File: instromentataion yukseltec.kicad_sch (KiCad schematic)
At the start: 0 parts

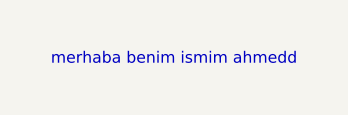
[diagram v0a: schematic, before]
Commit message: aa
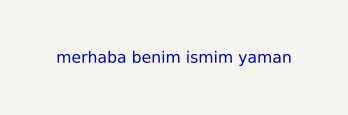
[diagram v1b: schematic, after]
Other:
- note added: "merhaba benim ismim yaman"
- note removed: "merhaba benim ismim ahmedd"
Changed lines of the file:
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@@
 	(generator_version "10.0")
 	(paper "A4")
-	(text "merhaba benim ismim ahmedd"
+	(text "merhaba benim ismim yaman"
 		(exclude_from_sim no)
 		(at 139.7 95.25 0)

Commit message: Revert "aa"
This reverts commit af853fb5f618a00eec8f8c9e7ae50b6d576ae841.
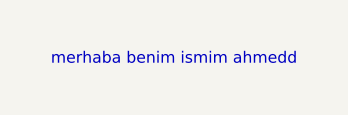
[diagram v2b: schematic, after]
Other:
- note added: "merhaba benim ismim ahmedd"
- note removed: "merhaba benim ismim yaman"
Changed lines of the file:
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@@
 	(generator_version "10.0")
 	(paper "A4")
-	(text "merhaba benim ismim yaman"
+	(text "merhaba benim ismim ahmedd"
 		(exclude_from_sim no)
 		(at 139.7 95.25 0)

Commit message: kardes_napyon_eklendi
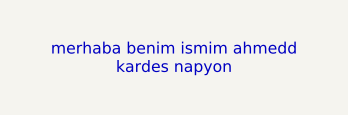
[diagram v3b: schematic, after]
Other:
- note added: "merhaba benim ismim ahmedd kardes napyon"
- note removed: "merhaba benim ismim ahmedd"
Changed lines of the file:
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@@
 	(generator_version "10.0")
 	(paper "A4")
-	(text "merhaba benim ismim ahmedd"
+	(text "merhaba benim ismim ahmedd\nkardes napyon"
 		(exclude_from_sim no)
 		(at 139.7 95.25 0)

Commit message: red_yedik
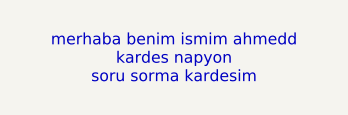
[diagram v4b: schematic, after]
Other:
- note added: "merhaba benim ismim ahmedd kardes napyon soru sorma kardesim"
- note removed: "merhaba benim ismim ahmedd kardes napyon"
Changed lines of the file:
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@@
 	(generator_version "10.0")
 	(paper "A4")
-	(text "merhaba benim ismim ahmedd\nkardes napyon"
+	(text "merhaba benim ismim ahmedd\nkardes napyon\nsoru sorma kardesim"
 		(exclude_from_sim no)
 		(at 139.7 95.25 0)

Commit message: ozur
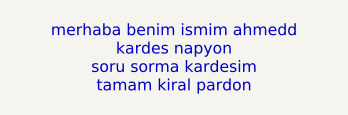
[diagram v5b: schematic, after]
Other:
- note added: "merhaba benim ismim ahmedd kardes napyon soru sorma kardesim tamam kiral pardon"
- note removed: "merhaba benim ismim ahmedd kardes napyon soru sorma kardesim"
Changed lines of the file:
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@@
 	(generator_version "10.0")
 	(paper "A4")
-	(text "merhaba benim ismim ahmedd\nkardes napyon\nsoru sorma kardesim"
+	(text "merhaba benim ismim ahmedd\nkardes napyon\nsoru sorma kardesim\ntamam kiral pardon"
 		(exclude_from_sim no)
 		(at 139.7 95.25 0)
